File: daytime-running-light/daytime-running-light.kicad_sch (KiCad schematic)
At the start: 61 parts, among them J1 Conn_01x02_Socket, J2 Conn_01x02_Socket, J3 Conn_01x01_Socket, J4 Conn_01x01_Socket, J5 Conn_01x01_Socket, J6 Conn_01x01_Pin, J7 Conn_01x01_Socket, Q1 IRF9540N, Q2 IRF9321, Q3 BC548, Q4 BC548, Q5 BC548, SW1 SW_SPST, SW2 SW_SPST, U1 L7812, U2 TLC555xP, U3 L7812, U4 4001, U5 4069

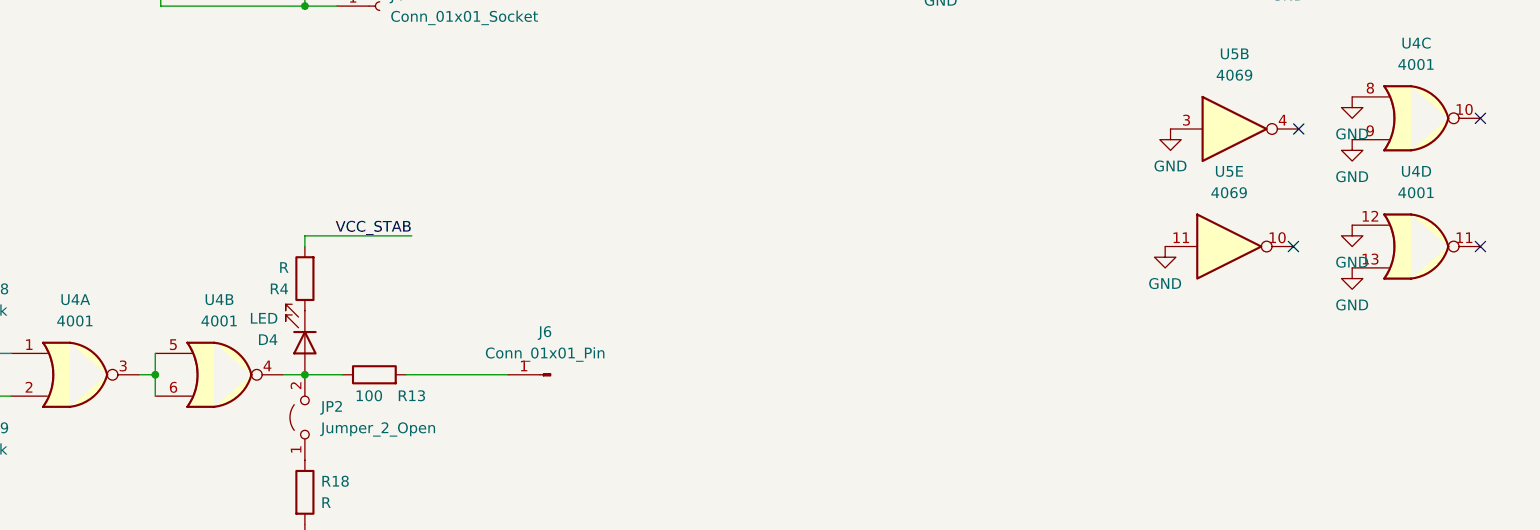
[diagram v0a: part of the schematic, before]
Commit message: [drl] Change schematic and PCB
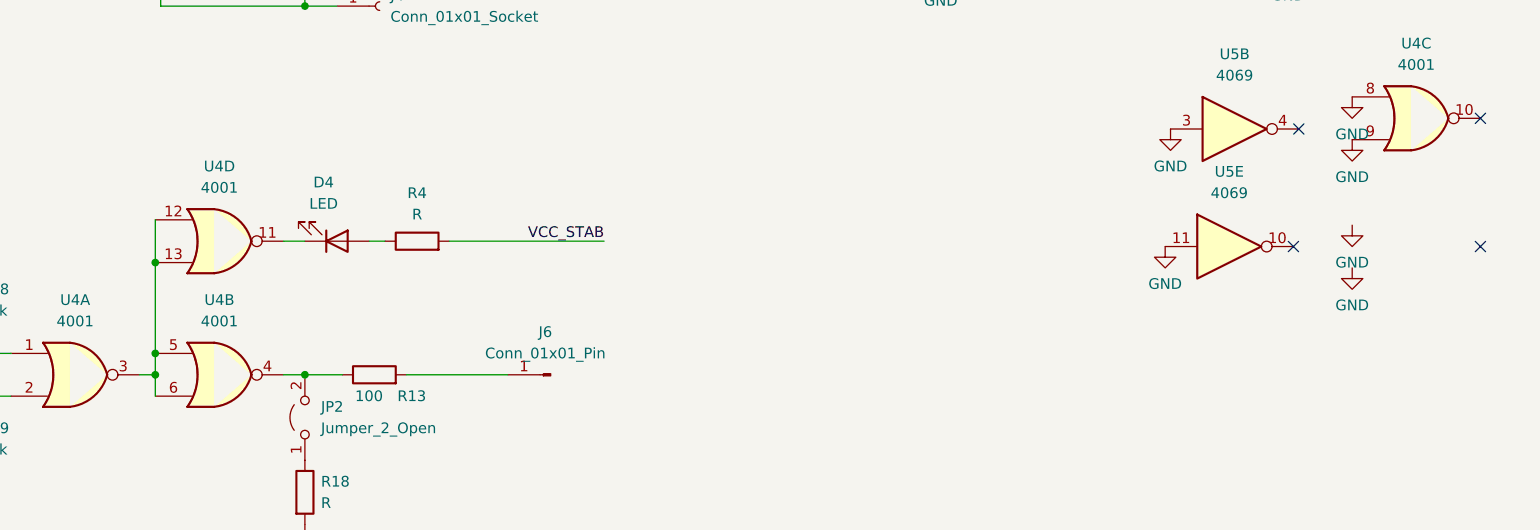
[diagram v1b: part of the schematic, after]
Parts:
- D4: footprint Connector_Wire:SolderWire-0.5sqmm_1x02_P4.6mm_D0.9mm_OD2.1mm -> LED_THT:LED_D5.0mm
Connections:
- net GND: no longer U4.12, U4.13
- net at U4.11: now also D4.1 (K)
- net at U4.3, U4.5, U4.6: now also U4.12, U4.13
- net at R4.1: now also D4.2 (A); no longer D4.1 (K)
- net at JP2.2 (B), R13.1, U4.4: no longer D4.2 (A)
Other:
- moved on the sheet: U4D
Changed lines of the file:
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@@
   (junction (at 55.88 113.03) (diameter 0) (color 0 0 0 0)
   )
+  (junction (at 120.015 168.275) (diameter 0) (color 0 0 0 0)
+  )
   (junction (at 59.69 155.575) (diameter 0) (color 0 0 0 0)
   )
@@
   )
   (junction (at 235.585 64.135) (diameter 0) (color 0 0 0 0)
+  )
+  (junction (at 120.015 157.48) (diameter 0) (color 0 0 0 0)
   )
   (junction (at 137.795 127) (diameter 0) (color 0 0 0 0)
@@
     (stroke (width 0) (type default))
   )
-  (wire (pts (xy 137.795 154.305) (xy 150.495 154.305))
-    (stroke (width 0) (type default))
-  )
   (wire (pts (xy 59.69 182.245) (xy 60.96 182.245))
     (stroke (width 0) (type default))
@@
     (stroke (width 0) (type default))
   )
-  (wire (pts (xy 137.795 154.305) (xy 137.795 155.575))
-    (stroke (width 0) (type default))
-  )
   (wire (pts (xy 120.015 170.815) (xy 120.015 168.275))
     (stroke (width 0) (type default))
@@
     (stroke (width 0) (type default))
   )
+  (wire (pts (xy 120.015 152.4) (xy 120.015 157.48))
+    (stroke (width 0) (type default))
+  )
   (wire (pts (xy 214.63 55.245) (xy 222.885 55.245))
     (stroke (width 0) (type default))
@@
     (stroke (width 0) (type default))
   )
+  (wire (pts (xy 120.015 157.48) (xy 120.015 168.275))
+    (stroke (width 0) (type default))
+  )
   (wire (pts (xy 137.795 120.65) (xy 137.795 127))
     (stroke (width 0) (type default))
@@
     (stroke (width 0) (type default))
   )
+  (wire (pts (xy 154.94 154.94) (xy 173.355 154.94))
+    (stroke (width 0) (type default))
+  )
   (wire (pts (xy 135.255 170.815) (xy 137.795 170.815))
     (stroke (width 0) (type default))
   )
+  (wire (pts (xy 145.415 154.94) (xy 147.32 154.94))
+    (stroke (width 0) (type default))
+  )
   (wire (pts (xy 101.6 57.15) (xy 101.6 62.23))
     (stroke (width 0) (type default))
@@
   )
   (wire (pts (xy 55.88 113.03) (xy 55.88 111.125))
+    (stroke (width 0) (type default))
+  )
+  (wire (pts (xy 135.255 154.94) (xy 137.795 154.94))
     (stroke (width 0) (type default))
   )
@@
     (effects (font (size 1.27 1.27)) (justify right bottom))
   )
+  (label "VCC_STAB" (at 173.355 154.94 180) (fields_autoplaced)
+    (effects (font (size 1.27 1.27)) (justify right bottom))
+  )
   (label "ALLOW_POWER_ON" (at 46.99 51.435 180) (fields_autoplaced)
     (effects (font (size 1.27 1.27)) (justify right bottom))
   )
   (label "VCC_STAB2" (at 20.955 23.495 270) (fields_autoplaced)
-    (effects (font (size 1.27 1.27)) (justify right bottom))
-  )
-  (label "VCC_STAB" (at 150.495 154.305 180) (fields_autoplaced)
     (effects (font (size 1.27 1.27)) (justify right bottom))
   )
@@
     )
   )
-  (symbol (lib_id "4xxx:4001") (at 269.875 155.575 0) (unit 4)
-    (in_bom yes) (on_board yes) (dnp no) (fields_autoplaced)
-    (property "Reference" "U4" (at 269.875 146.685 0)
-      (effects (font (size 1.27 1.27)))
-    )
-    (property "Value" "4001" (at 269.875 149.225 0)
-      (effects (font (size 1.27 1.27)))
-    )
-    (property "Footprint" "Package_DIP:DIP-14_W7.62mm" (at 269.875 155.575 0)
-      (effects (font (size 1.27 1.27)) hide)
-    )
-    (property "Datasheet" "http://www.intersil.com/content/dam/Intersil/documents/cd40/cd4000bms-01bms-02bms-25bms.pdf" (at 269.875 155.575 0)
+  (symbol (lib_id "4xxx:4001") (at 127.635 154.94 0) (unit 4)
+    (in_bom yes) (on_board yes) (dnp no) (fields_autoplaced)
+    (property "Reference" "U4" (at 127.635 146.05 0)
+      (effects (font (size 1.27 1.27)))
+    )
+    (property "Value" "4001" (at 127.635 148.59 0)
+      (effects (font (size 1.27 1.27)))
+    )
+    (property "Footprint" "Package_DIP:DIP-14_W7.62mm" (at 127.635 154.94 0)
+      (effects (font (size 1.27 1.27)) hide)
+    )
+    (property "Datasheet" "http://www.intersil.com/content/dam/Intersil/documents/cd40/cd4000bms-01bms-02bms-25bms.pdf" (at 127.635 154.94 0)
       (effects (font (size 1.27 1.27)) hide)
     )
@@
     )
   )
+  (symbol (lib_id "Device:R") (at 151.13 154.94 90) (unit 1)
+    (in_bom yes) (on_board yes) (dnp no) (fields_autoplaced)
+    (property "Reference" "R4" (at 151.13 149.225 90)
+      (effects (font (size 1.27 1.27)))
+    )
+    (property "Value" "R" (at 151.13 151.765 90)
+      (effects (font (size 1.27 1.27)))
+    )
+    (property "Footprint" "Resistor_THT:R_Axial_DIN0207_L6.3mm_D2.5mm_P2.54mm_Vertical" (at 151.13 156.718 90)
+      (effects (font (size 1.27 1.27)) hide)
+    )
+    (property "Datasheet" "~" (at 151.13 154.94 0)
+      (effects (font (size 1.27 1.27)) hide)
+    )
+    (pin "1")
+    (pin "2")
+    (instances
+      (project "daytime-running-light"
+        (path "/f8c2c6dd-d5ef-40d1-be2c-9a93444b1d43"
+          (reference "R4") (unit 1)
+        )
+      )
+    )
+  )
   (symbol (lib_id "power:GND") (at 213.36 121.285 0) (unit 1)
     (in_bom yes) (on_board yes) (dnp no) (fields_autoplaced)
@@
     )
   )
-  (symbol (lib_id "Device:R") (at 137.795 159.385 180) (unit 1)
-    (in_bom yes) (on_board yes) (dnp no) (fields_autoplaced)
-    (property "Reference" "R4" (at 135.89 160.655 0)
-      (effects (font (size 1.27 1.27)) (justify left))
-    )
-    (property "Value" "R" (at 135.89 158.115 0)
-      (effects (font (size 1.27 1.27)) (justify left))
-    )
-    (property "Footprint" "Resistor_THT:R_Axial_DIN0207_L6.3mm_D2.5mm_P2.54mm_Vertical" (at 139.573 159.385 90)
-      (effects (font (size 1.27 1.27)) hide)
-    )
-    (property "Datasheet" "~" (at 137.795 159.385 0)
-      (effects (font (size 1.27 1.27)) hide)
-    )
-    (pin "1")
-    (pin "2")
-    (instances
-      (project "daytime-running-light"
-        (path "/f8c2c6dd-d5ef-40d1-be2c-9a93444b1d43"
-          (reference "R4") (unit 1)
-        )
-      )
-    )
-  )
   (symbol (lib_id "power:GND") (at 262.255 137.795 0) (unit 1)
     (in_bom yes) (on_board yes) (dnp no) (fields_autoplaced)
@@
     )
   )
+  (symbol (lib_id "Device:LED") (at 141.605 154.94 0) (mirror x) (unit 1)
+    (in_bom yes) (on_board yes) (dnp no)
+    (property "Reference" "D4" (at 140.0175 147.955 0)
+      (effects (font (size 1.27 1.27)))
+    )
+    (property "Value" "LED" (at 140.0175 150.495 0)
+      (effects (font (size 1.27 1.27)))
+    )
+    (property "Footprint" "LED_THT:LED_D5.0mm" (at 141.605 154.94 0)
+      (effects (font (size 1.27 1.27)) hide)
+    )
+    (property "Datasheet" "~" (at 141.605 154.94 0)
+      (effects (font (size 1.27 1.27)) hide)
+    )
+    (pin "1")
+    (pin "2")
+    (instances
+      (project "daytime-running-light"
+        (path "/f8c2c6dd-d5ef-40d1-be2c-9a93444b1d43"
+          (reference "D4") (unit 1)
+        )
+      )
+    )
+  )
   (symbol (lib_id "Device:C_Polarized") (at 135.255 33.02 0) (unit 1)
     (in_bom yes) (on_board yes) (dnp no) (fields_autoplaced)
@@
         )
       )
-    )
-  )
-  (symbol (lib_id "Device:LED") (at 137.795 167.005 270) (unit 1)
-    (in_bom yes) (on_board yes) (dnp no) (fields_autoplaced)
-    (property "Reference" "D4" (at 134.62 166.6875 90)
-      (effects (font (size 1.27 1.27)) (justify right))
-    )
-    (property "Value" "LED" (at 134.62 164.1475 90)
-      (effects (font (size 1.27 1.27)) (justify right))
-    )
-    (property "Footprint" "Connector_Wire:SolderWire-0.5sqmm_1x02_P4.6mm_D0.9mm_OD2.1mm" (at 137.795 167.005 0)
-      (effects (font (size 1.27 1.27)) hide)
-    )
-    (property "Datasheet" "~" (at 137.795 167.005 0)
-      (effects (font (size 1.27 1.27)) hide)
-    )
-    (pin "1")
-    (pin "2")
-    (instances
-      (project "daytime-running-light"
-        (path "/f8c2c6dd-d5ef-40d1-be2c-9a93444b1d43"
-          (reference "D4") (unit 1)
-        )
-      )
